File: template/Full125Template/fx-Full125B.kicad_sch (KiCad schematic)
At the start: 1 part, among them J101 Conn_01x08_Pin

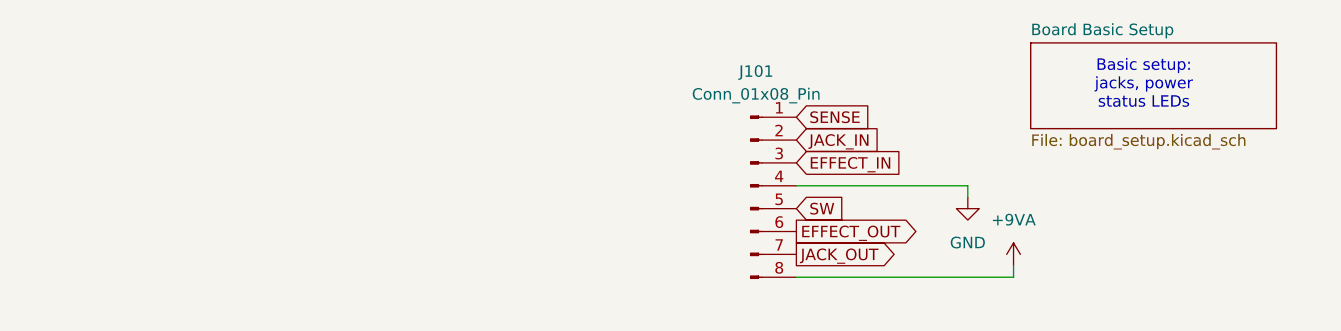
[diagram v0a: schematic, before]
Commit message: Update Full 125B template
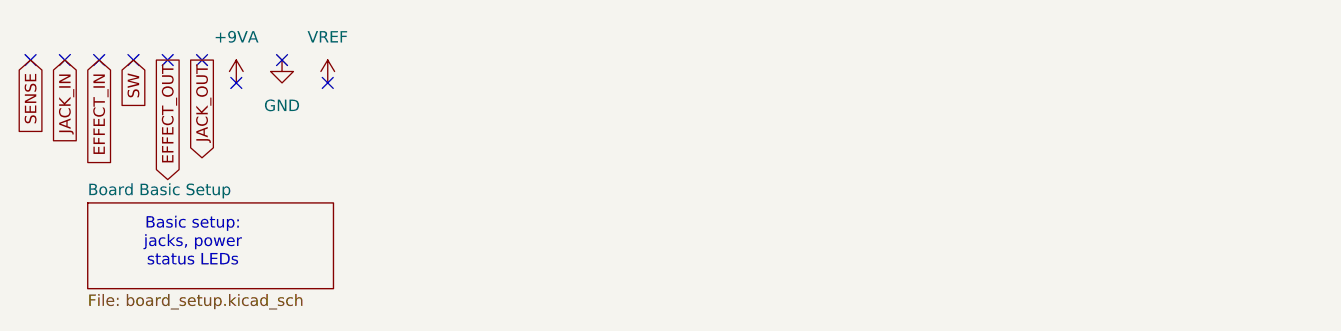
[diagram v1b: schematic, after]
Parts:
- removed J101: Conn_01x08_Pin, Connector_PinSocket_2.54mm:PinSocket_1x08_P2.54mm_Vertical, symbol Connector:Conn_01x08_Pin
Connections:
- no-connect marks 0 -> 9
